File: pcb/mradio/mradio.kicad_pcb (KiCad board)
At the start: 6 copper layers, 132.2 x 75 mm, 191 parts, among them J101 Conn_02x07_Odd_Even, J202 Conn_01x02, J301 2250065-1, J401 MM60-52B1-E1-R650, J501 MDT420E01001, Q101 Q_NMOS, Q102 Q_NMOS, Q103 Q_NMOS, Q104 Q_NMOS, Q105 Q_NMOS, Q106 Q_NMOS, Q107 Q_NMOS, Q108 Q_NMOS, Q301 SSM3K56FS_LF, U1 STM32H745ZITx, U301 DP83825I, U401 74AVC4T774, U402 74AVC4T774, U502 SN74LVC1T45DRL, U601 TPS54560BDDA, U701 TPS54560BDDA, U801 TPS7A8500ARGRR, U901 TPS7A8500ARGRR, Y301 DSC1525JL2A-25M00000T

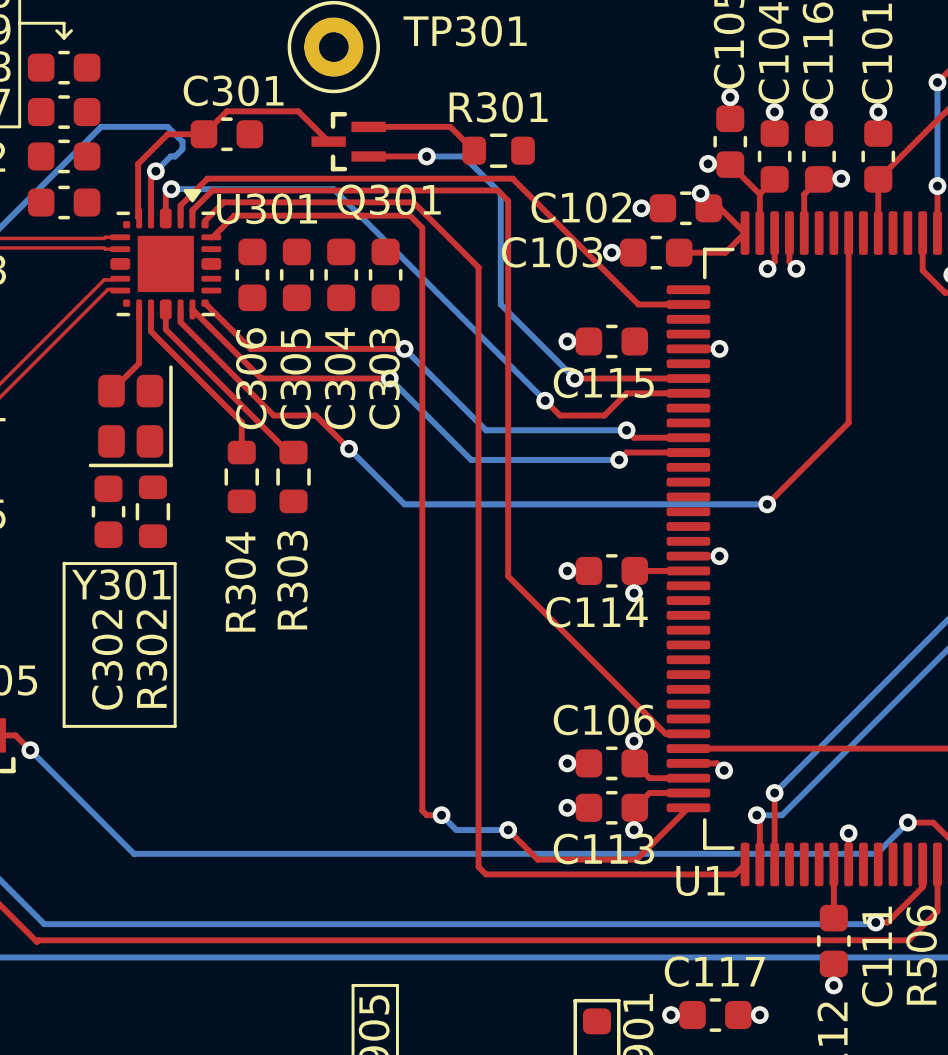
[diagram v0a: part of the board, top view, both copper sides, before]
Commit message: eth changes
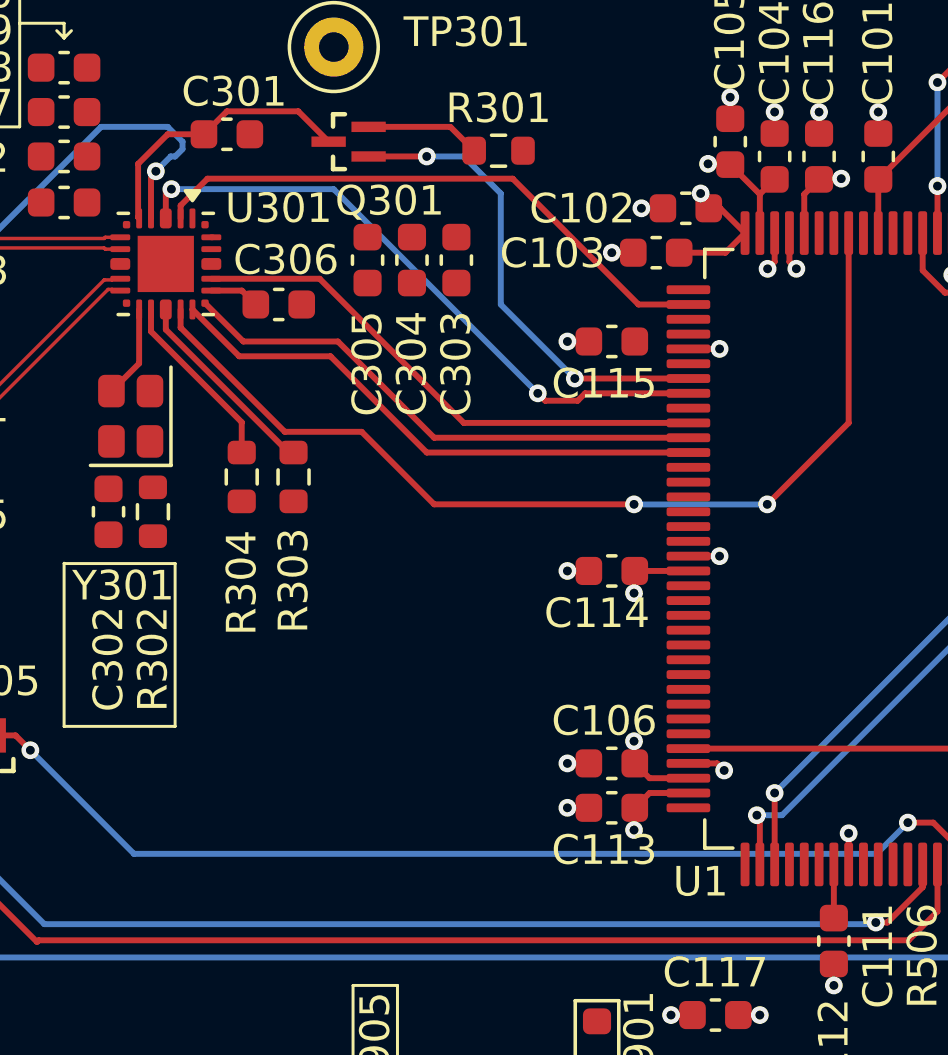
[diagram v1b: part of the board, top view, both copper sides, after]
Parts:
- moved C303 2.44 mm to (92.5, 62.5)
- moved C304 2.44 mm to (91.0, 62.5)
- moved C305 2.44 mm to (89.5, 62.5)
- moved C306 1.34 mm to (86.5, 64.0), turned to 180 degrees
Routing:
- net ETH_TXD1: track 40.0 -> 0.00 mm
- net ETH_TXD0: track 37.7 -> 0.05 mm, vias 2 -> 0
- net ETH_TX_EN: track 32.3 -> 0.00 mm
- net ETH_CRS_DV: track 0.00 -> 18.1 mm
- net +1V8: track 71.2 -> 72.9 mm
- net ETH_RXD1: track 19.0 -> 18.8 mm, vias 2 -> 0
- net ETH_RXD0: vias 2 -> 0
